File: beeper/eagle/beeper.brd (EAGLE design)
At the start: 27.6 x 41.9 mm, 32 parts, among them Q1 16MHz, T1 3904, U1 ATMEGA328P, U2 ATA6631

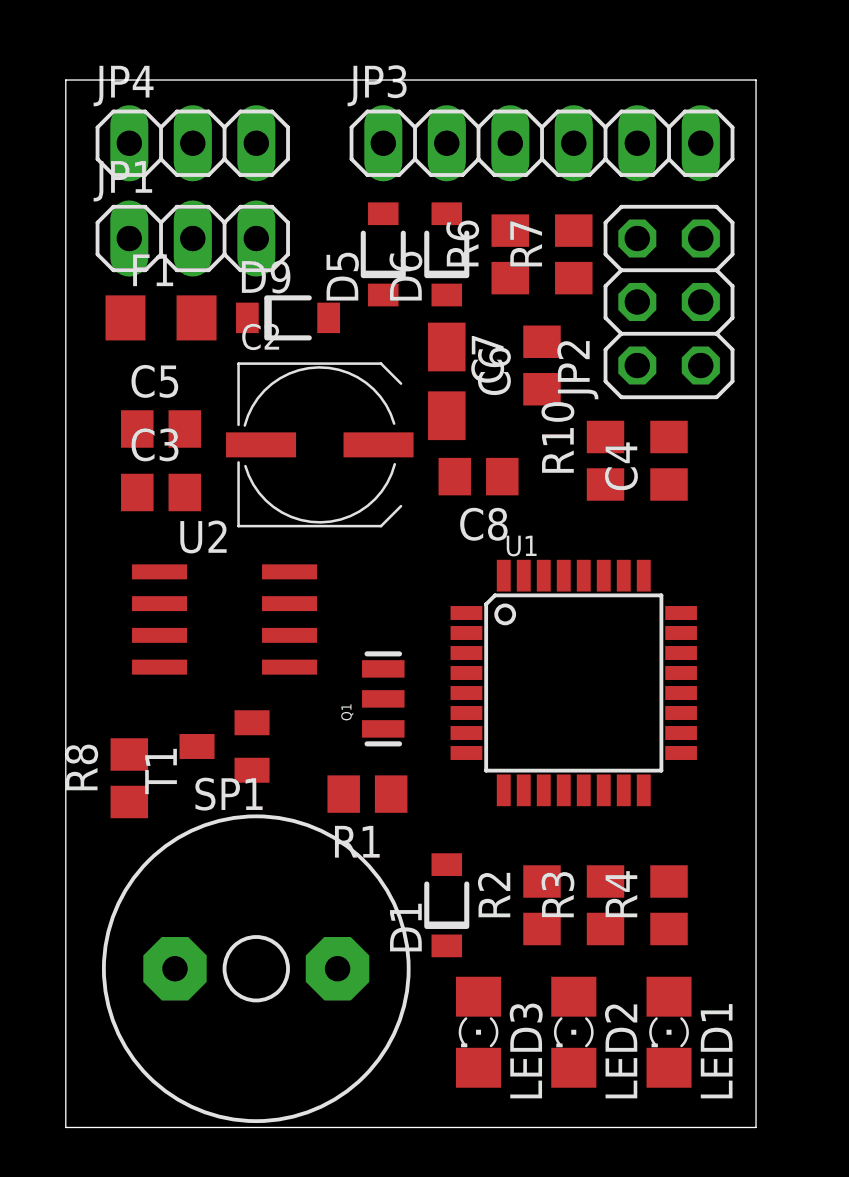
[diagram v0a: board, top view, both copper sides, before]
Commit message: Minor board tweaks. Work in progress.
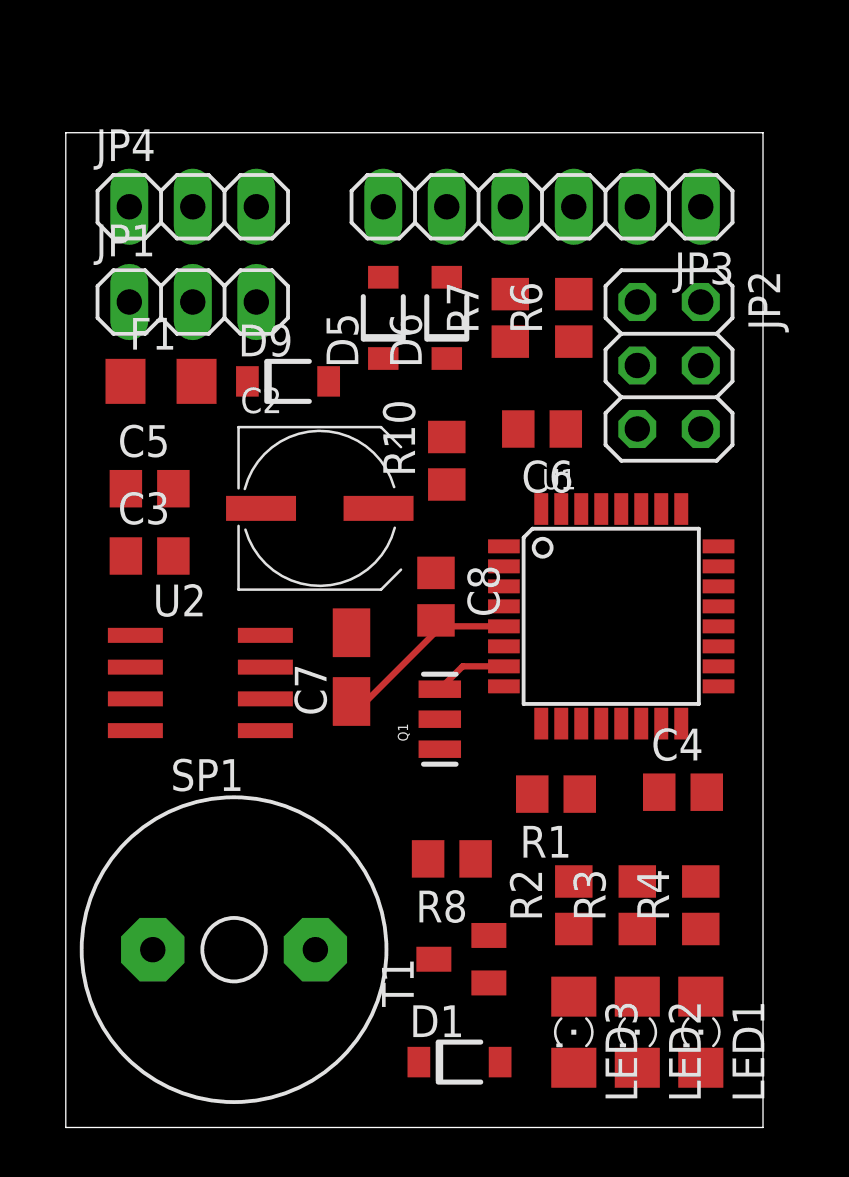
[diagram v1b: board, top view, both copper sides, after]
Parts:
- moved R8 13.3 mm to (15.4, 10.7), turned to 180 degrees
- moved C4 13.3 mm to (24.7, 13.4), turned to 0 degrees
- moved T1 12.7 mm to (15.8, 6.73)
- moved C7 12.0 mm to (11.4, 18.4), turned to 90 degrees
- moved R1 7.54 mm to (19.6, 13.3)
- moved R10 6.35 mm to (15.2, 26.7)
- moved D1 6.29 mm to (15.7, 2.62), turned to 0 degrees
- moved C8 5.09 mm to (14.8, 21.2), turned to 270 degrees
- moved LED3 3.81 mm to (20.3, 3.81)
- moved R6 3.59 mm to (20.3, 32.4)
- moved R7 3.59 mm to (17.8, 32.4)
- moved U1 3.06 mm to (21.8, 20.4)
- moved U2 2.72 mm to (5.38, 17.8)
- moved C3 2.58 mm to (3.35, 22.9)
- moved JP2 2.54 mm to (24.1, 30.5), turned to 270 degrees
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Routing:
- net GND: track 0.00 -> 7.18 mm
- net N$1: track 0.00 -> 2.94 mm
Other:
- board size 27.6 x 41.9 mm -> 27.9 x 39.8 mm
